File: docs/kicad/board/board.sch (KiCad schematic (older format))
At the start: 17 parts, among them J1 VIN, J10 WHEEL_4, J11 FLAG, J12 LED, J13 COMPASS, J14 SWITCH, J2 LEFT, J3 RIGHT, J4 UNUSED, J5 ARM, J6 LID, J7 WHEEL_1, J8 WHEEL_2, J9 WHEEL_3, SW1 BUTTON_1, SW2 BUTTON_2, U1 ARDUINO_NANO

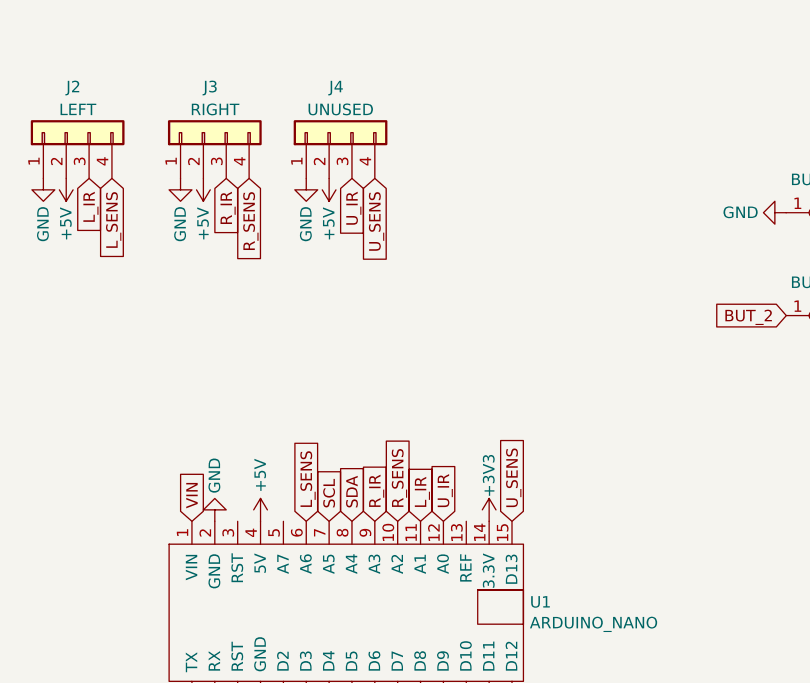
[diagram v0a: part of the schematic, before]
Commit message: Built version 2 for Daniel
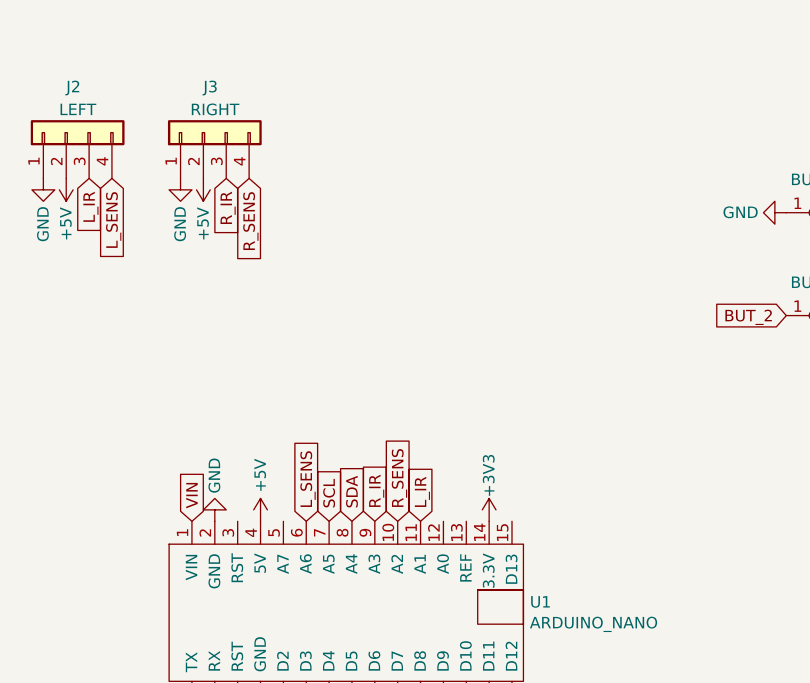
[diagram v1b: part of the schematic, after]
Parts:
- removed J4: UNUSED, cnc3018-PCB:my4pin, symbol Connector_Generic:Conn_01x04
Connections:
- net U_IR: no longer names the net of U1.12 (A0)
- net U_SENS: no longer names the net of U1.15 (D13)
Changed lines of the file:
@@
 Text GLabel 4850 3050 1    50   Input ~ 0
 R_IR
-Text GLabel 5150 3050 1    50   Input ~ 0
-U_IR
 Text GLabel 4550 3050 1    50   Input ~ 0
 L_SENS
 Text GLabel 4950 3050 1    50   Input ~ 0
 R_SENS
-Text GLabel 5450 3050 1    50   Input ~ 0
-U_SENS
 Text GLabel 4650 3850 3    50   Input ~ 0
 WHEEL_1
@@
 	-1   0    0    1
 $EndComp
-$Comp
-L Connector_Generic:Conn_01x04 J4
-U 1 1 63300773
-P 4650 1350
-F 0 "J4" V 4850 1350 50  0000 R CNN
-F 1 "UNUSED" V 4750 1300 50  0000 C CNN
-F 2 "cnc3018-PCB:my4pin" H 4650 1350 50  0001 C CNN
-F 3 "~" H 4650 1350 50  0001 C CNN
-	1    4650 1350
-	0    -1   -1   0
-$EndComp
-$Comp
-L power:GND #PWR06
-U 1 1 63300779
-P 4550 1550
-F 0 "#PWR06" H 4550 1300 50  0001 C CNN
-F 1 "GND" V 4550 1350 50  0000 C CNN
-F 2 "" H 4550 1550 50  0001 C CNN
-F 3 "" H 4550 1550 50  0001 C CNN
-	1    4550 1550
-	1    0    0    -1
-$EndComp
-$Comp
-L power:+5V #PWR07
-U 1 1 6330077F
-P 4650 1550
-F 0 "#PWR07" H 4650 1400 50  0001 C CNN
-F 1 "+5V" V 4650 1750 50  0000 C CNN
-F 2 "" H 4650 1550 50  0001 C CNN
-F 3 "" H 4650 1550 50  0001 C CNN
-	1    4650 1550
-	-1   0    0    1
-$EndComp
 Text GLabel 3700 1550 3    50   Input ~ 0
 L_SENS
-Text GLabel 4850 1550 3    50   Input ~ 0
-U_SENS
 Text GLabel 4300 1550 3    50   Input ~ 0
 R_SENS
 Text GLabel 3600 1550 3    50   Input ~ 0
 L_IR
-Text GLabel 4750 1550 3    50   Input ~ 0
-U_IR
 Text GLabel 4200 1550 3    50   Input ~ 0
 R_IR
